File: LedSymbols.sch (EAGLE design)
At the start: 17 parts, among them IC1 PIC16F628P

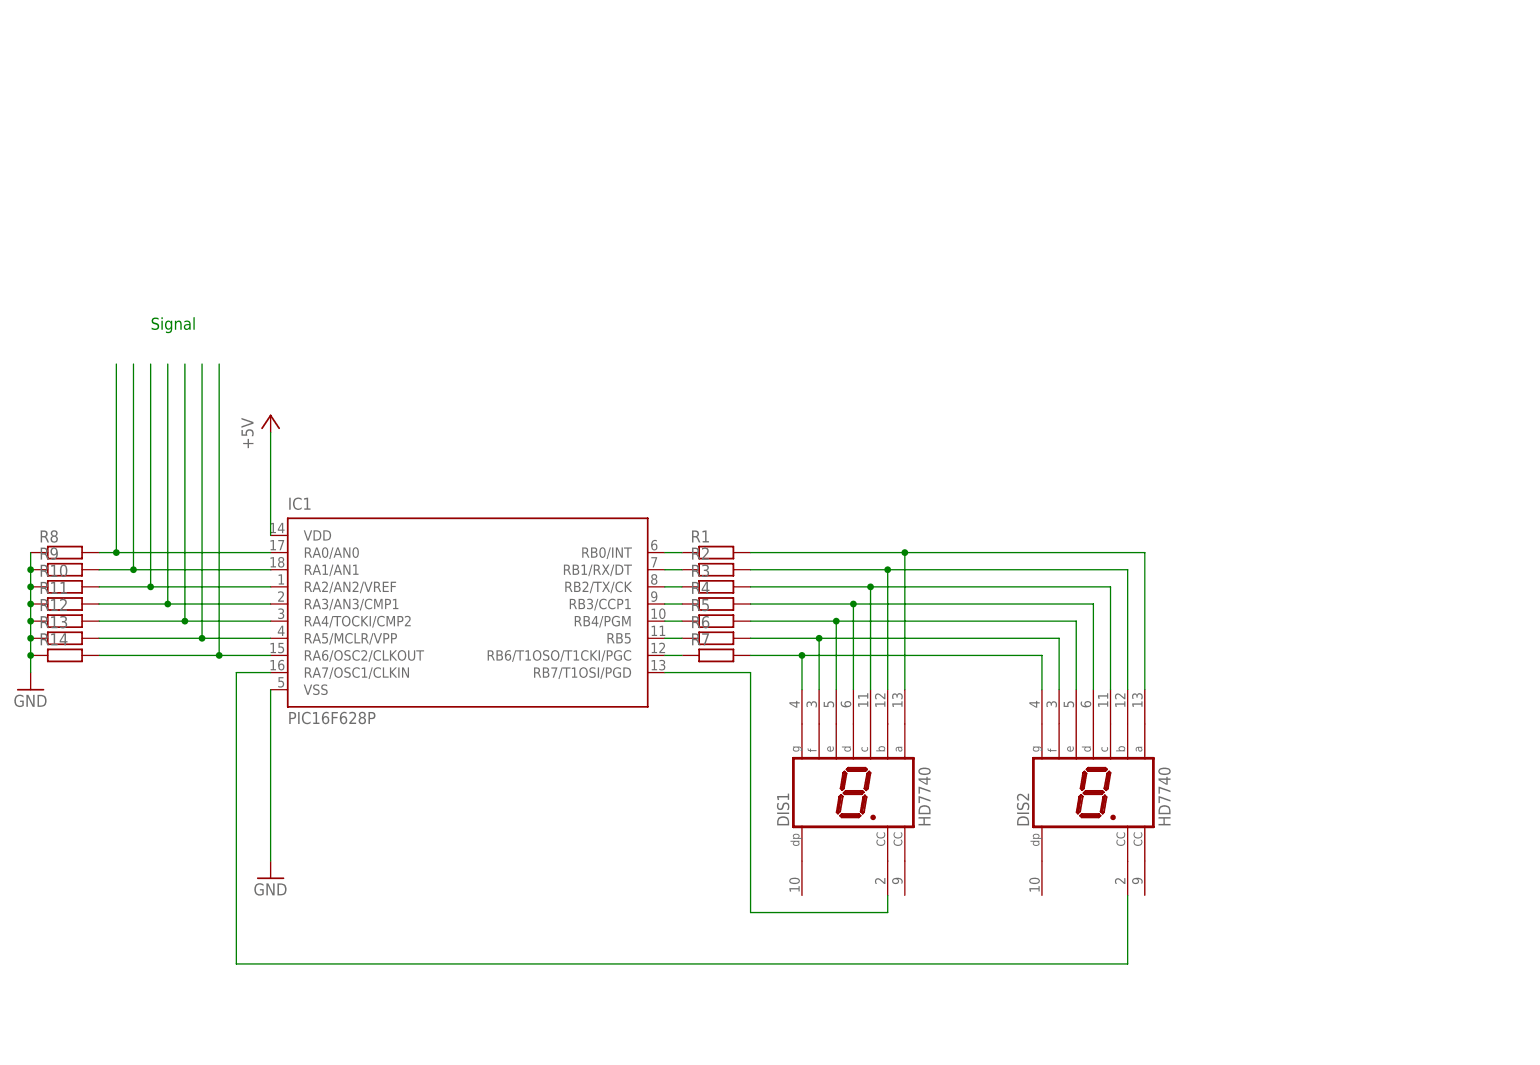
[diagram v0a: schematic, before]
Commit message: Updating scheme
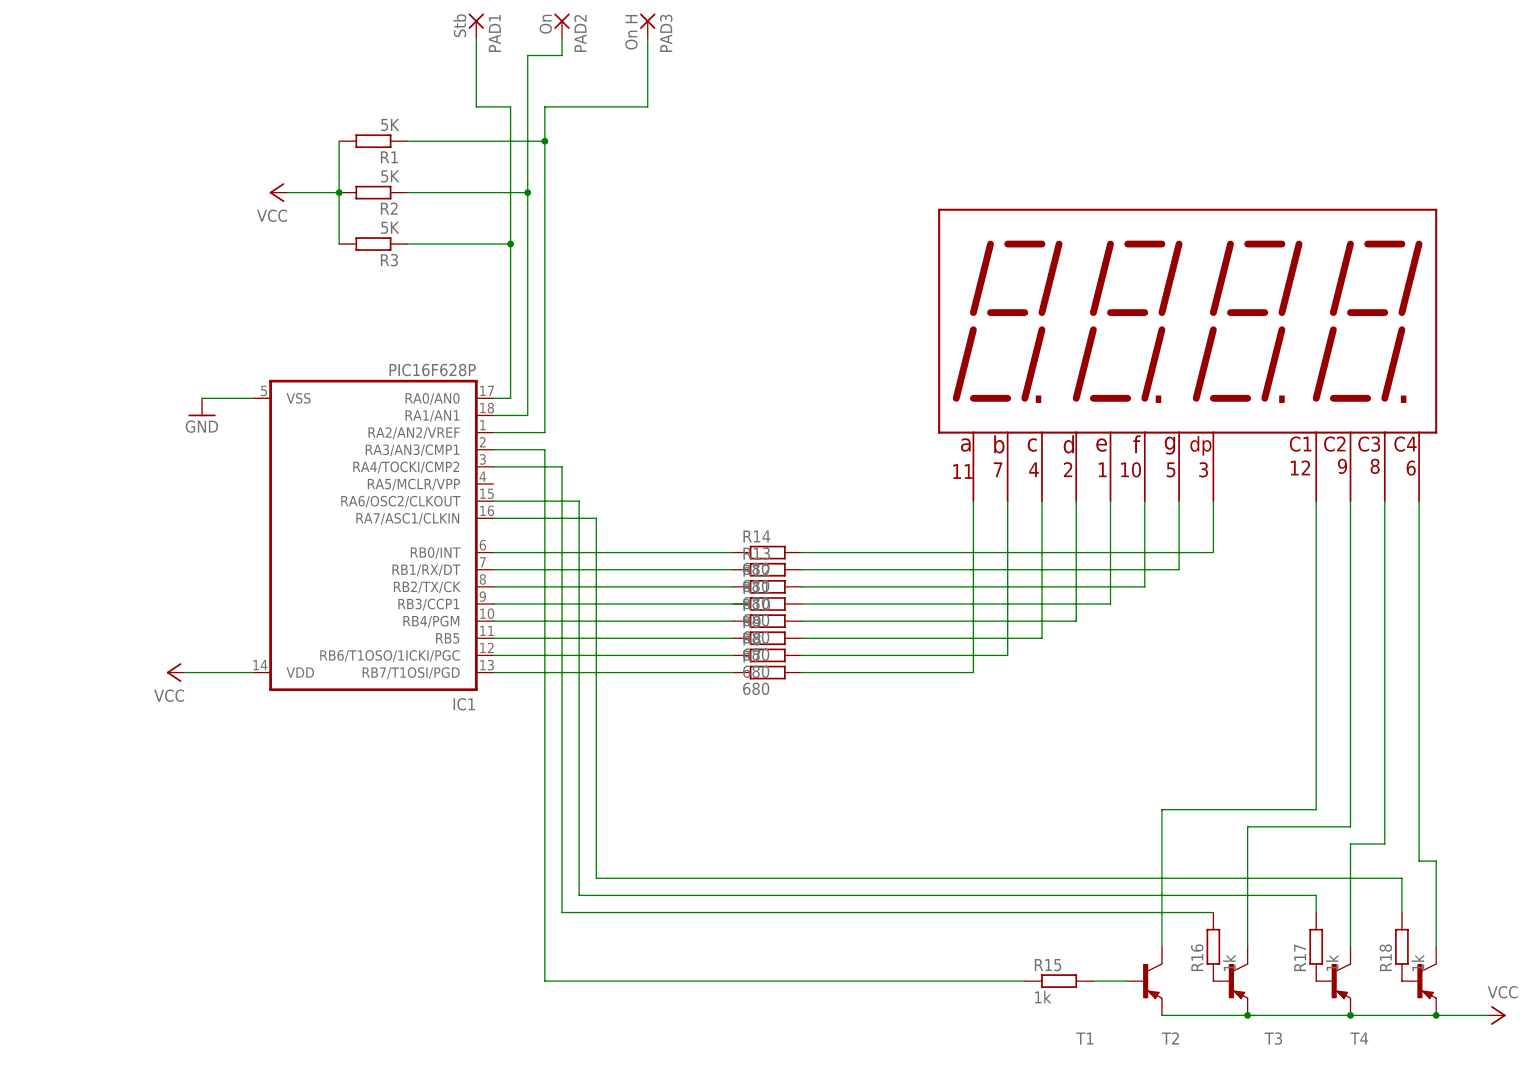
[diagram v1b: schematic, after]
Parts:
- removed DIS1, DIS2: HD7740, display-hp:HD7740
- removed R4, R5, R6: (no value), rcl:R-EU_0207/7
- added PAD1: Stb, wirepad:1,6/0,8
- added PAD2: On, wirepad:1,6/0,8
- added PAD3: On H, wirepad:1,6/0,8
- added R15, R16, R17, R18: 1k, rcl:R-EU_0207/10
- added T1, T2, T3, T4: (no value), transistor:BC327-16-PNP-TO92-EBC
- added U$2: 7SEGM, 1-mano-bibl:7SEGM
- R1, R2, R3: value (none) -> 5K; device rcl:R-EU_0207/7 -> rcl:R-EU_0207/10
- R10, R11, R12, R13, R14, R7, R8, R9: value (none) -> 680; device rcl:R-EU_0207/7 -> rcl:R-EU_0207/10
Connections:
- removed net +5V: IC1.VDD
- removed net N$25: IC1.RA4/TOCKI/CMP2, R12.2
- removed net N$26: IC1.RA5/MCLR/VPP, R13.2
- removed net N$27: IC1.RA6/OSC2/CLKOUT, R14.2
- removed net N$28: IC1.RA0/AN0, R8.2
- new net N$15: R14.2
- new net N$16: R15.2, T1.B
- new net N$17: R16.1, T2.B
- new net N$18: R17.1, T3.B
- new net N$19: R18.1, T4.B
- new net N$35: IC1.RA7/ASC1/CLKIN, R18.2
- new net N$37: IC1.RA4/TOCKI/CMP2, R16.2
- new net N$38: IC1.RA3/AN3/CMP1, R15.1
- new net N$43: T1.C
- new net N$44: T2.C
- new net N$45: T3.C
- new net N$46: T4.C
- new net VCC: IC1.VDD, R1.2, R2.2, R3.2, T1.E, T2.E, T3.E, T4.E
- net GND: no longer R10.1, R11.1, R12.1, R13.1, R14.1, R8.1, R9.1
- net N$1: now also IC1.RB0/INT, R14.1; no longer DIS1.G, DIS2.G, R7.2
- net N$10: now also R9.2; no longer IC1.RB2/TX/CK, R3.1
- net N$11: now also R10.2; no longer IC1.RB3/CCP1, R4.1
- net N$12: now also R11.2; no longer IC1.RB4/PGM, R5.1
- net N$13: now also R12.2; no longer IC1.RB5, R6.1
- net N$14: now also R13.2; no longer IC1.RB6/T1OSO/T1CKI/PGC, R7.1
- net N$2: now also IC1.RB1/RX/DT, R13.1; no longer DIS1.F, DIS2.F, R6.2
- net N$20: now also R7.1; no longer DIS1.CC
- net N$21: now also IC1.RA0/AN0, PAD1.P, R3.1; no longer DIS2.CC, IC1.RA7/OSC1/CLKIN
- net N$22: now also PAD2.P, R2.1; no longer R9.2
- net N$23: now also PAD3.P, R1.1; no longer R10.2
- net N$24: now also IC1.RA6/OSC2/CLKOUT, R17.2; no longer IC1.RA3/AN3/CMP1, R11.2
- net N$3: now also IC1.RB2/TX/CK, R12.1; no longer DIS1.E, DIS2.E, R5.2
- net N$4: now also IC1.RB3/CCP1; no longer DIS1.D, DIS2.D, R4.2
- net N$5: now also IC1.RB4/PGM, R10.1; no longer DIS1.C, DIS2.C, R3.2
- net N$6: now also IC1.RB5, R9.1; no longer DIS1.B, DIS2.B, R2.2
- net N$7: now also IC1.RB6/T1OSO/1ICKI/PGC, R8.1; no longer DIS1.A, DIS2.A, R1.2
- net N$8: now also R7.2; no longer IC1.RB0/INT, R1.1
- net N$9: now also R8.2; no longer IC1.RB1/RX/DT, R2.1
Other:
- note removed: "Signal"
- moved on the sheet: IC1, R1, R10, R11, R12, R13, R14, R2, R3, R7, R8, R9
